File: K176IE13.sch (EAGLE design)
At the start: 103 parts, among them J1 0R-JUMPB

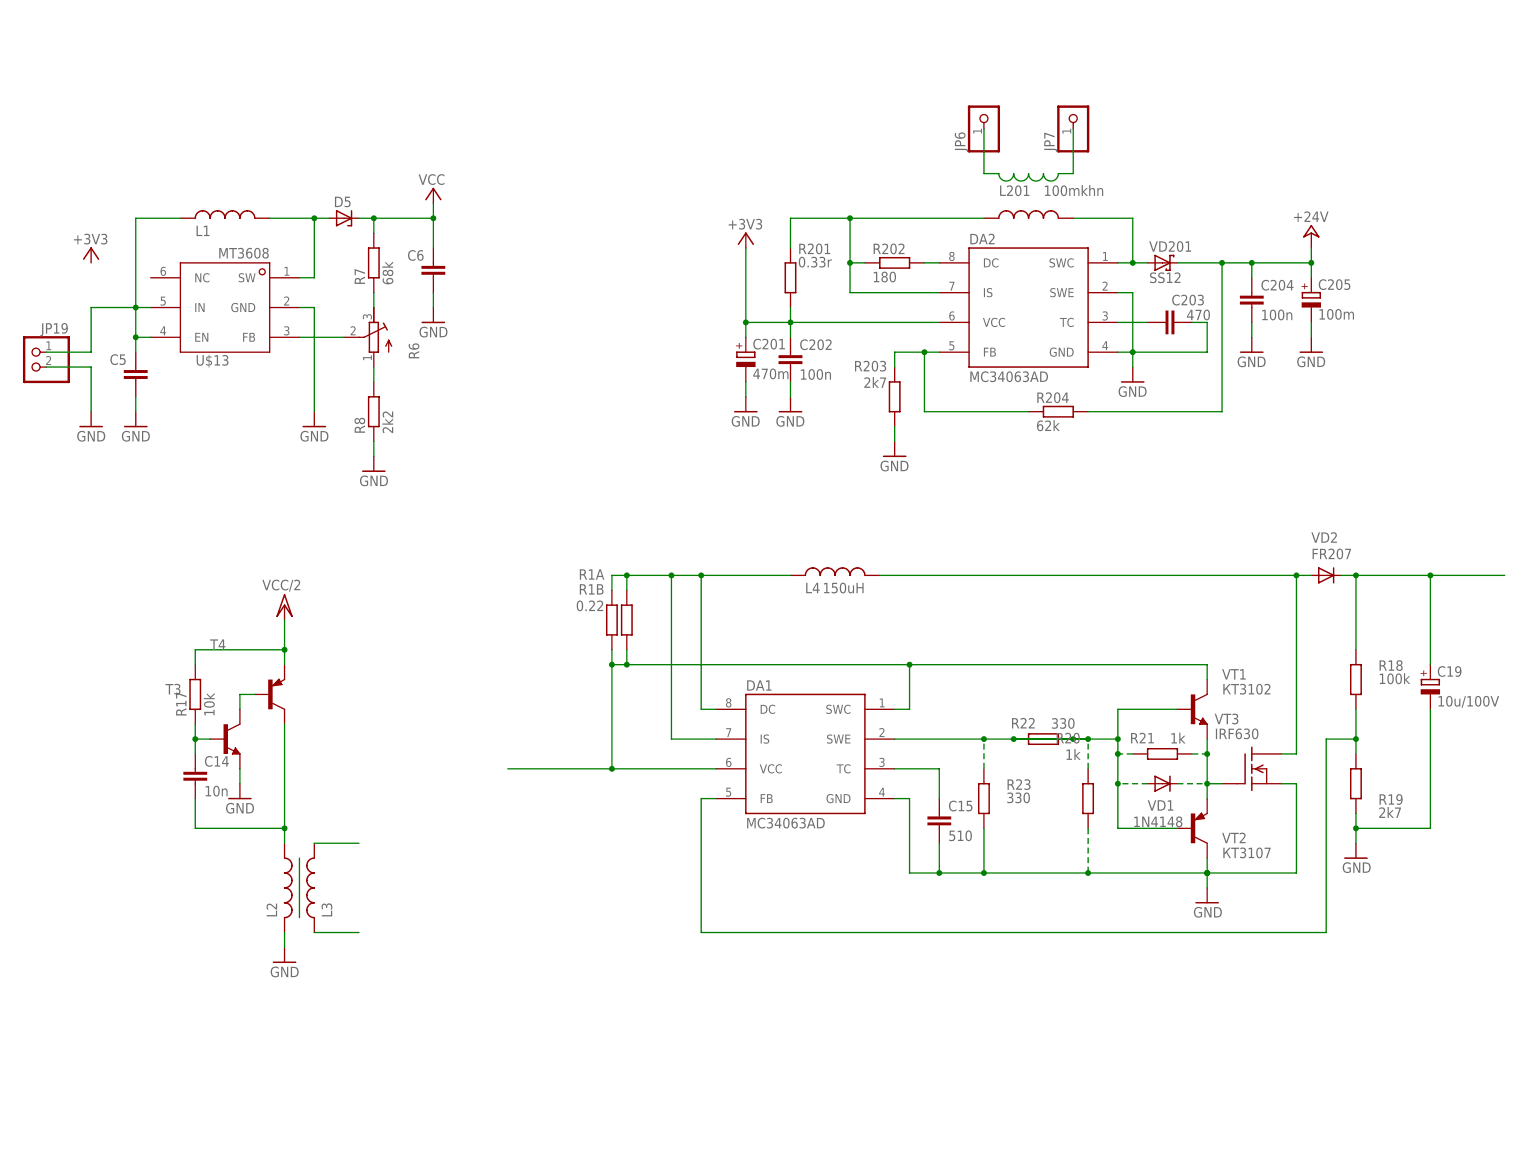
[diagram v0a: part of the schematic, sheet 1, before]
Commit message: .
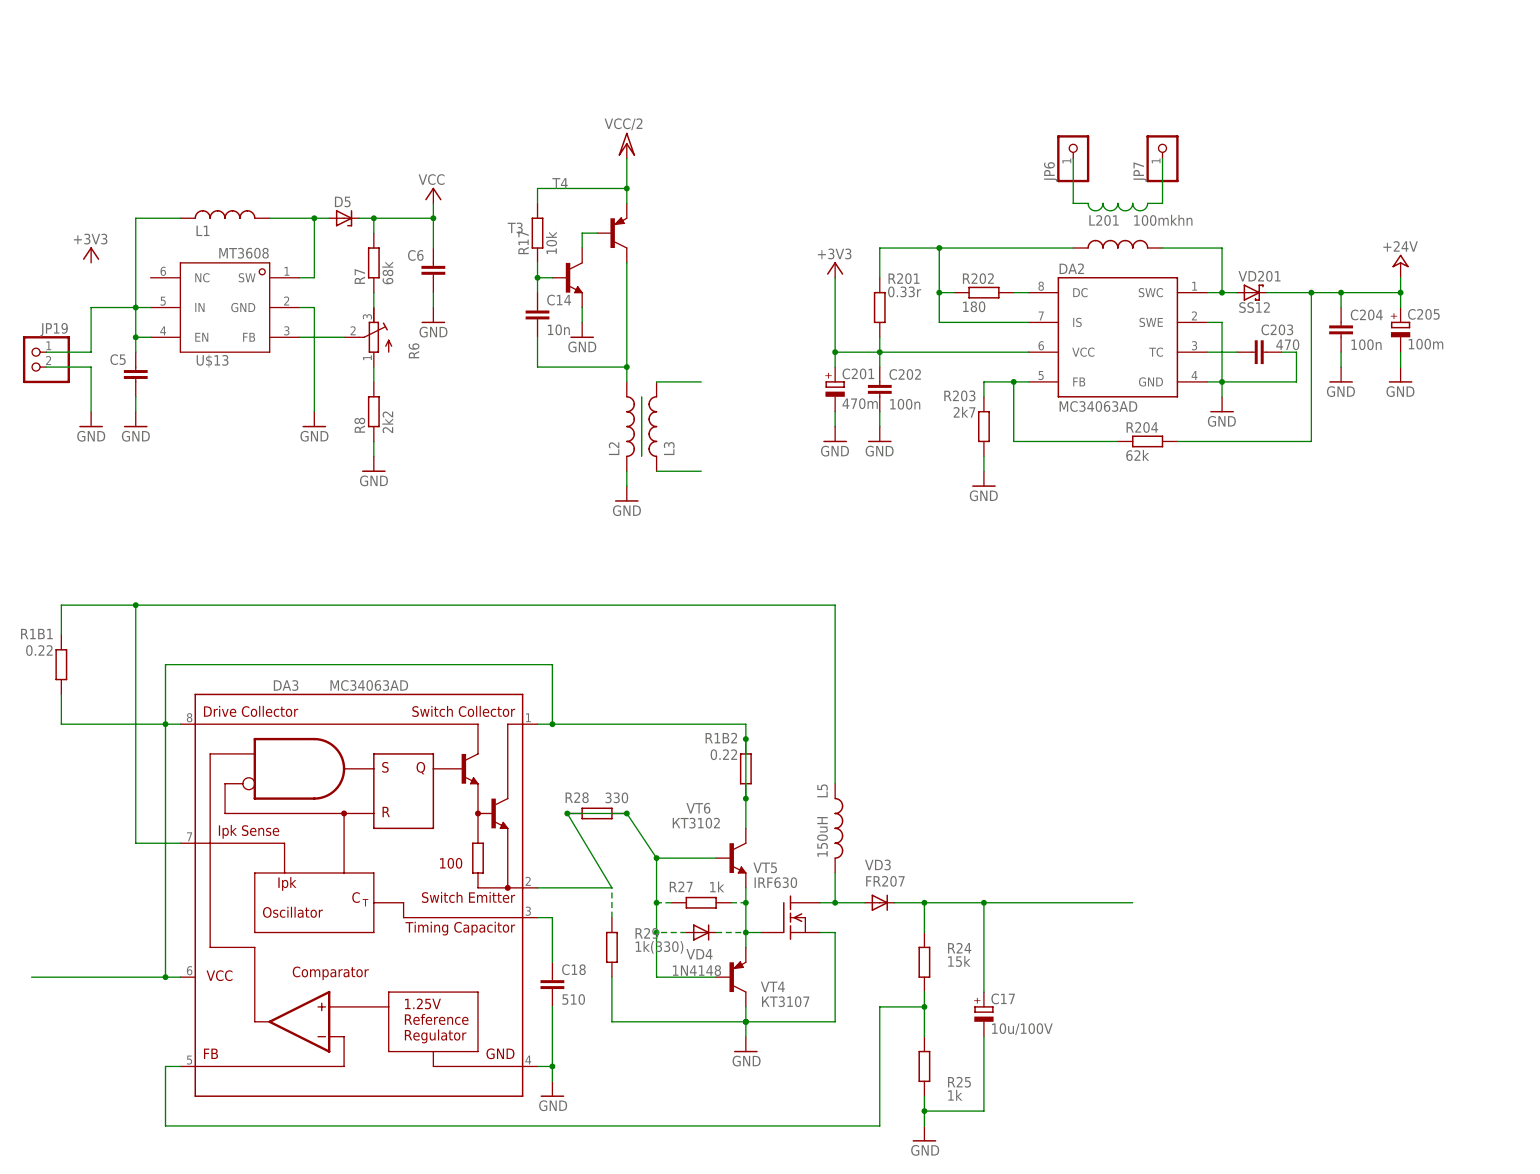
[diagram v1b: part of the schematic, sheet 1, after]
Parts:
- removed C15: 510, resistor:C-EUC0805K
- removed C19: 10u/100V, rcl:CPOL-EUTT5D9L
- removed DA1: MC34063AD, mc34063-2:MC34063AD
- removed L4: 150uH, rcl:L-US0204/7
- removed R18: 100k, rcl:R-EU_R0805
- removed R19: 2k7, rcl:R-EU_R0805
- removed R1A: (no value), resistor:R-EU_R1206
- removed R1B: 0.22, resistor:R-EU_R1206
- removed R20, R21: 1k, rcl:R-EU_R0805
- removed R22, R23: 330, rcl:R-EU_R0805
- removed VD1: 1N4148, diode:DIODE-SOD80C
- removed VD2: FR207, diode:DIODE-DO41-10
- removed VT1: КТ3102, transistor-npn:BC338
- removed VT2: КТ3107, transistor-pnp:MPSA64
- removed VT3: IRF630, transistor-fet:BUZ22
- added C17: 10u/100V, rcl:CPOL-EUTT5D9L
- added C18: 510, resistor:C-EUC0805K
- added DA3: MC34063AD, mc34063:MC34063TAD
- added L5: 150uH, rcl:L-US0204/7
- added R1B1, R1B2: 0.22, resistor:R-EU_R1206
- added R24: 15k, rcl:R-EU_R0805
- added R25, R27: 1k, rcl:R-EU_R0805
- added R28: 330, rcl:R-EU_R0805
- added R29: 1k(330), rcl:R-EU_R0805
- added VD3: FR207, diode:DIODE-DO41-10
- added VD4: 1N4148, diode:DIODE-SOD80C
- added VT4: КТ3107, transistor-pnp:MPSA64
- added VT5: IRF630, transistor-fet:BUZ22
- added VT6: КТ3102, transistor-npn:BC338
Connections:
- removed net N$77: DA1.SWE, R20.1, R21.1, R22.1, R22.2, R23.2, VD1.A, VT1.B, VT2.B
- removed net N$83: C15.1, DA1.TC
- removed net N$87: L4.2, VD2.A, VT3.D
- removed net N$89: DA1.FB, R18.1, R19.2
- removed net N$90: C19.+, R18.2, VD2.C
- removed net N$95: R21.2, VD1.C, VT1.E, VT2.E, VT3.G
- new net N$79: DA3.SWE, R27.1, R28.1, R28.2, R29.2, VD4.A, VT4.B, VT6.B
- new net N$88: L5.2, VD3.A, VT5.D
- new net N$91: DA3.FB, R24.1, R25.2
- new net N$94: DA3.IS, L5.1, R1B1.2
- new net N$96: DA3.DC, DA3.SWC, DA3.VCC, R1B1.1, R1B2.1, R1B2.2, VT6.C
- new net N$98: C18.1, DA3.TC
- net GND: now also C17.-, C18.2, DA3.GND, R25.1, R29.1, VT4.C, VT5.S; no longer C15.2, C19.-, DA1.GND, R19.1, R20.2, R23.1, VT2.C, VT3.S
- net N$92: now also C17.+, R24.2, VD3.C; no longer DA1.SWC, DA1.VCC, R1A.1, R1B.1, VT1.C
- net N$93: now also R27.2, VD4.C, VT4.E, VT5.G, VT6.E; no longer DA1.DC, DA1.IS, L4.1, R1A.2, R1B.2
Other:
- moved on the sheet: C14, C201, C202, C203, C204, C205, DA2, JP6, JP7, L2, L201, L3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
